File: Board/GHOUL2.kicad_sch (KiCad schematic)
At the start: 16 parts, among them J1 Conn_01x02, Q1 IRF540N, Q2 IRF540N, U1 Teensy3.5_All_Pins, U10 GHOULIMU, U2 LM7805_TO220, U3 BMP280, U4 Feedback_Serv, U5 LM1084-ADJ, U6 NichromeConnector, U7 Ultimate_GPS_Breakout_v3, U8 Xbee, U9 NichromeConnector

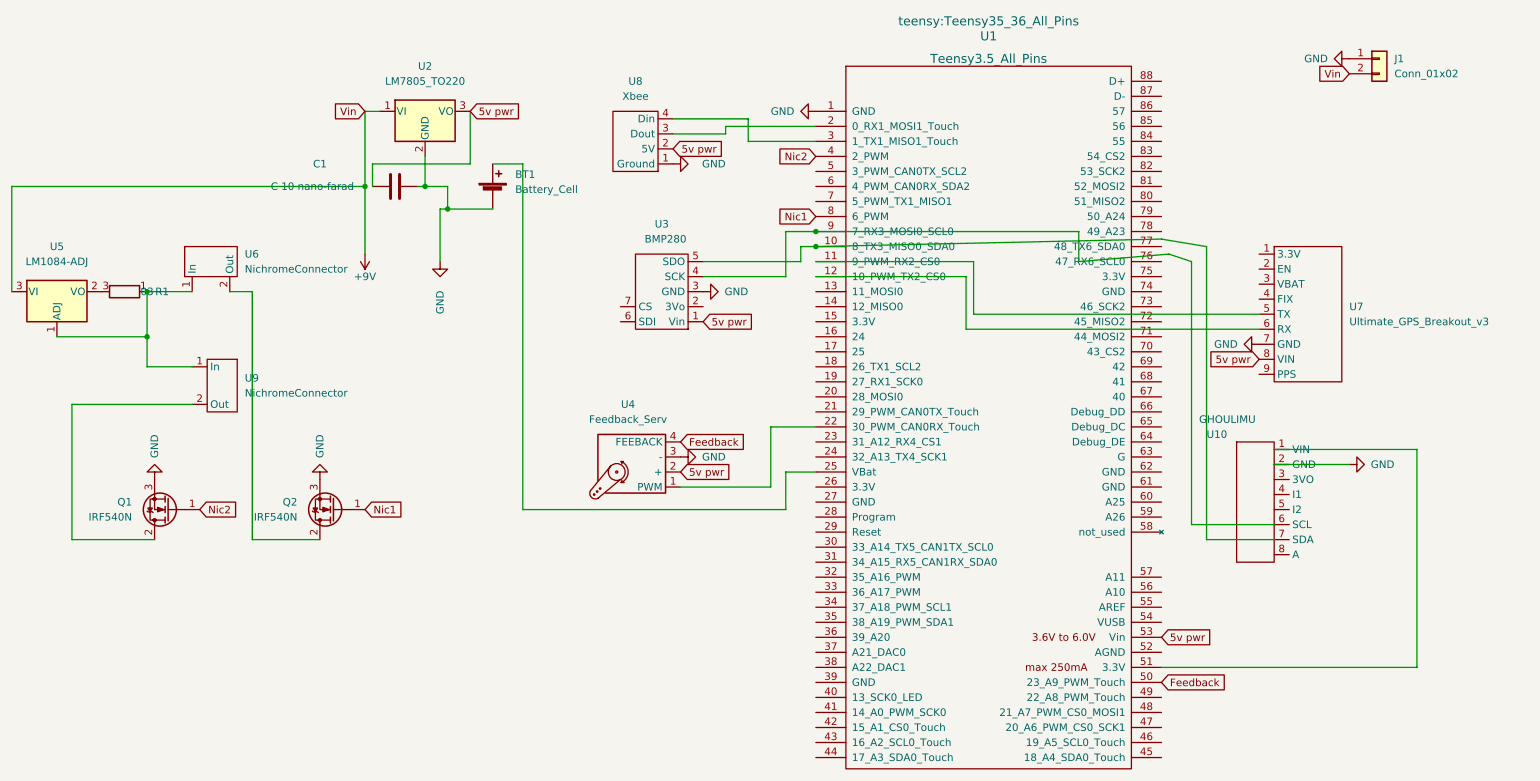
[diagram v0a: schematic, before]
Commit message: lots of improvements
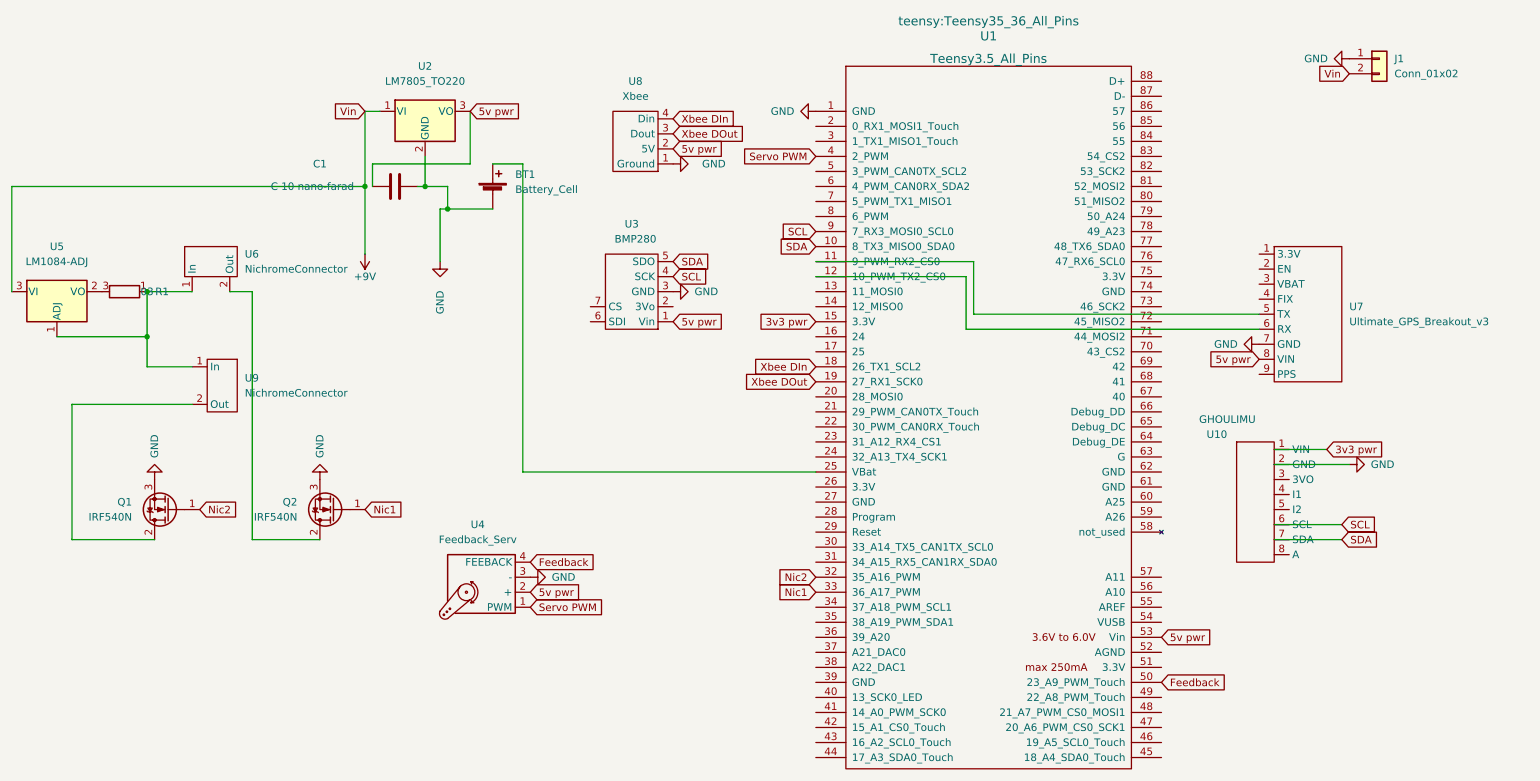
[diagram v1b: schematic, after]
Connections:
- net Nic1: now also U1.33 (36_A17_PWM); no longer U1.8 (6_PWM)
- net Nic2: now also U1.32 (35_A16_PWM); no longer U1.4 (2_PWM)
- net at U1.22 (30_PWM_CAN0RX_Touch): no longer U4.1 (PWM)
- net at U1.2 (0_RX1_MOSI1_Touch): no longer U8.3 (Dout)
- net at U1.3 (1_TX1_MISO1_Touch): no longer U8.4 (Din)
- net SCL: now reaches U1.9 (7_RX3_MOSI0_SCL0), U10.6 (SCL), U3.4 (SCK)
- net SDA: now reaches U1.10 (8_TX3_MISO0_SDA0), U10.7 (SDA), U3.5 (SDO)
- net 3v3 pwr: now reaches U1.15 (3.3V)
- net 3v3 pwr: now also U10.1 (VIN)
- net Xbee DIn: now reaches U1.18 (26_TX1_SCL2)
- net Xbee DIn: now also U8.4 (Din)
- net Xbee DOut: now reaches U1.19 (27_RX1_SCK0)
- net Xbee DOut: now also U8.3 (Dout)
- net at U1.51 (3.3V): no longer U10.1 (VIN)
- new net Servo PWM: U1.4 (2_PWM), U4.1 (PWM)
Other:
- moved on the sheet: U3, U4

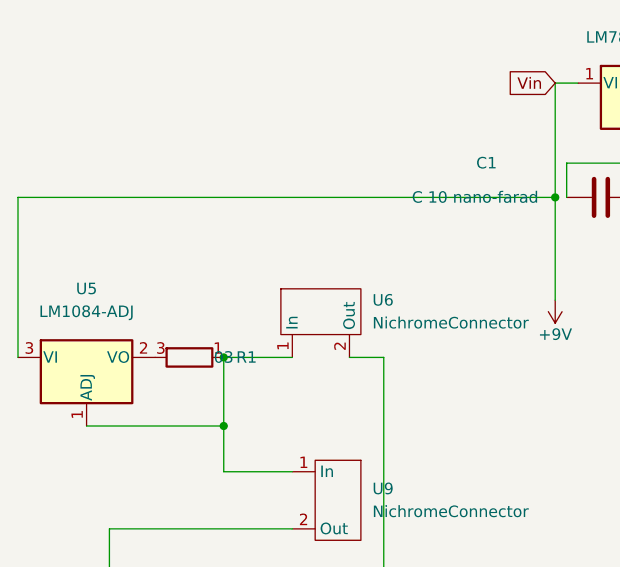
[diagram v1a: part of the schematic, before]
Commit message: for real this time... ?
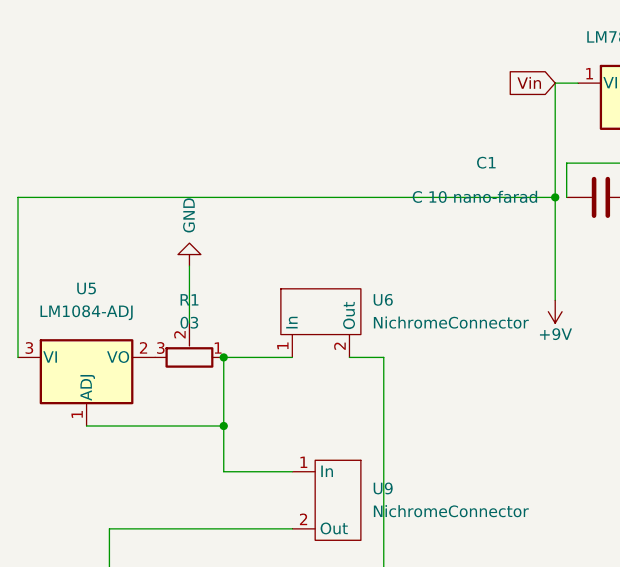
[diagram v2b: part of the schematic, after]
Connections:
- net GND: now also R1.2
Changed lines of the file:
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@@
+    (stroke (width 0) (type default) (color 0 0 0 0))
+  )
+  (wire (pts (xy 55.88 60.96) (xy 55.88 67.31))
     (stroke (width 0) (type default) (color 0 0 0 0))
   )
@@
   (symbol (lib_id "Device:R") (at 55.88 71.12 270) (unit 1)
     (in_bom yes) (on_board yes) (fields_autoplaced)
-    (property "Reference" "R1" (id 0) (at 62.23 71.12 90))
-    (property "Value" "03" (id 1) (at 59.69 71.12 90))
-    (property "Footprint" "Package_TO_SOT_SMD:TO-263-2" (id 2) (at 57.658 71.12 90)
+    (property "Reference" "R1" (id 0) (at 55.88 64.77 90))
+    (property "Value" "03" (id 1) (at 55.88 67.31 90))
+    (property "Footprint" "Package_TO_SOT_SMD:TO-263-2" (id 2) (at 55.88 69.342 90)
       (effects (font (size 1.27 1.27)) hide)
     )
@@
     )
     (pin "1")
+    (pin "2")
     (pin "3")
   )
@@
     )
     (property "Datasheet" "" (id 3) (at 148.59 49.53 0)
+      (effects (font (size 1.27 1.27)) hide)
+    )
+    (pin "1")
+  )
+  (symbol (lib_id "power:GND") (at 55.88 60.96 180) (unit 1)
+    (in_bom yes) (on_board yes)
+    (property "Reference" "#PWR0112" (id 0) (at 55.88 54.61 0)
+      (effects (font (size 1.27 1.27)) hide)
+    )
+    (property "Value" "GND" (id 1) (at 55.88 53.34 90)
+      (effects (font (size 1.27 1.27)) (justify left))
+    )
+    (property "Footprint" "" (id 2) (at 55.88 60.96 0)
+      (effects (font (size 1.27 1.27)) hide)
+    )
+    (property "Datasheet" "" (id 3) (at 55.88 60.96 0)
       (effects (font (size 1.27 1.27)) hide)
     )
@@
       (reference "#PWR0111") (unit 1) (value "GND") (footprint "")
     )
+    (path "/c766f8cf-c139-4fb1-afd5-9c039f651864"
+      (reference "#PWR0112") (unit 1) (value "GND") (footprint "")
+    )
     (path "/e100fb02-ae0f-4575-a8f0-e7fb3c16a01e"
